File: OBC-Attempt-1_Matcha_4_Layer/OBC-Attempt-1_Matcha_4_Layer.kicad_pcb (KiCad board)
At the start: 4 copper layers, 57.1 x 57.1 mm, 76 parts, among them J1 Screw_Terminal_01x08, J2 Screw_Terminal_01x08, J3 USB_B_Micro, J4 Screw_Terminal_01x08, J5 Conn_01x04, J6 Micro_SD_Card, J7 Screw_Terminal_01x02, J8 Screw_Terminal_01x02, Q1 2N7002K, Q2 2N7002K, Q3 2N7002K, Q4 2N7002K, SW1 PCM12SMTR, U1 BMI088, U10 CPC1020NTR, U11 CPC1020NTR, U12 NCP1117-3.3_SOT223, U2 CPC1020NTR, U3 CPC1020NTR, U4 CPC1020NTR, U5 CPC1020NTR, U6 NCP1117-3.3_SOT223, U7 CPC1020NTR, U8 CPC1020NTR, U9 STM32F401RDTx, Y1 ABMM2-25MHZ-D1-T

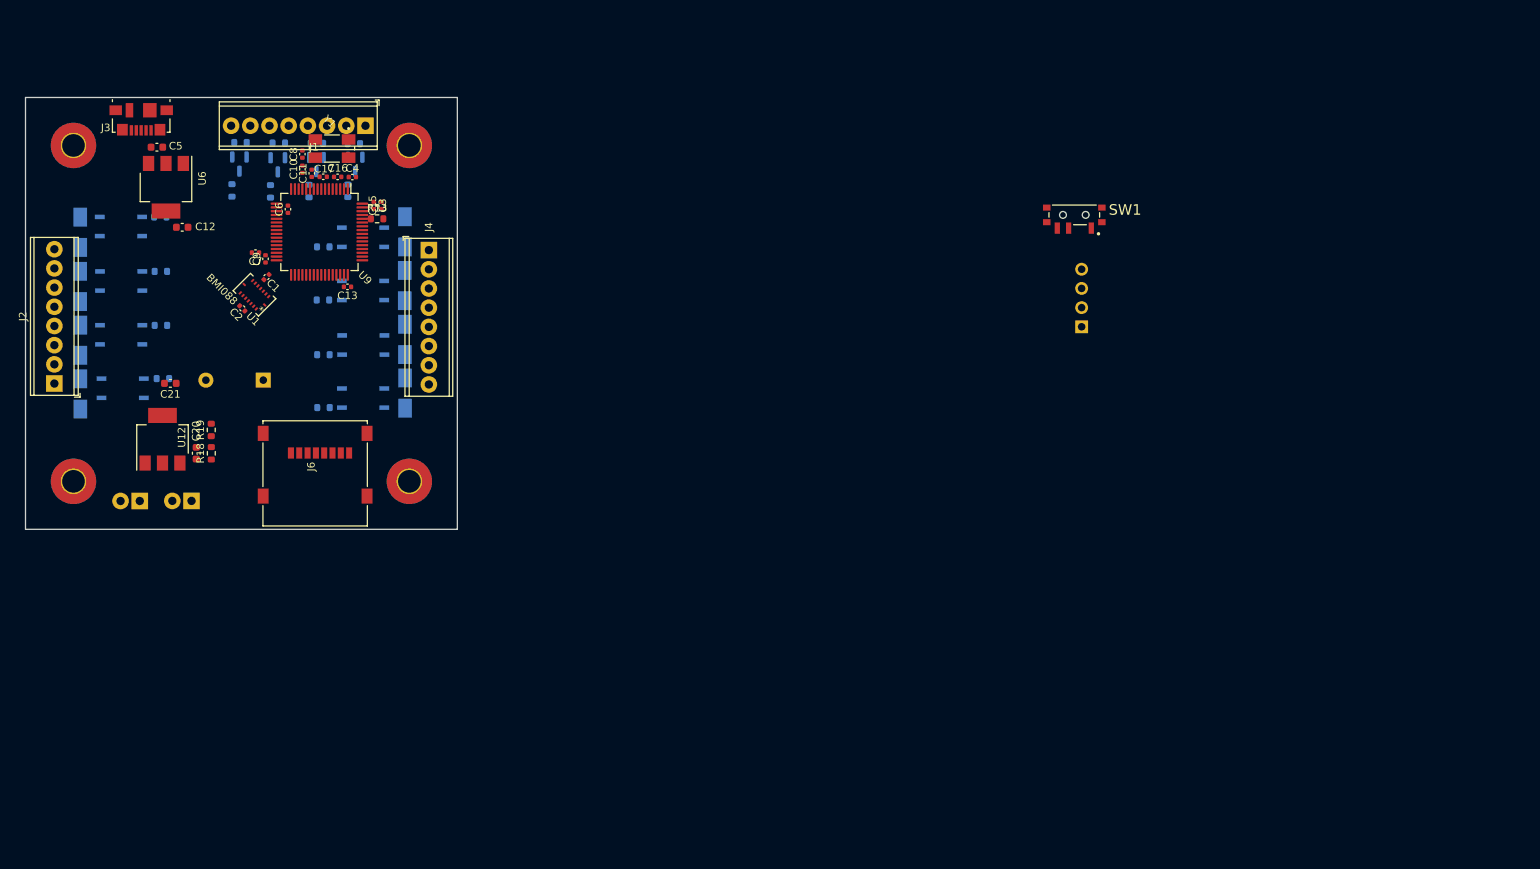
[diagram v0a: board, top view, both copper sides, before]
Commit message: start over
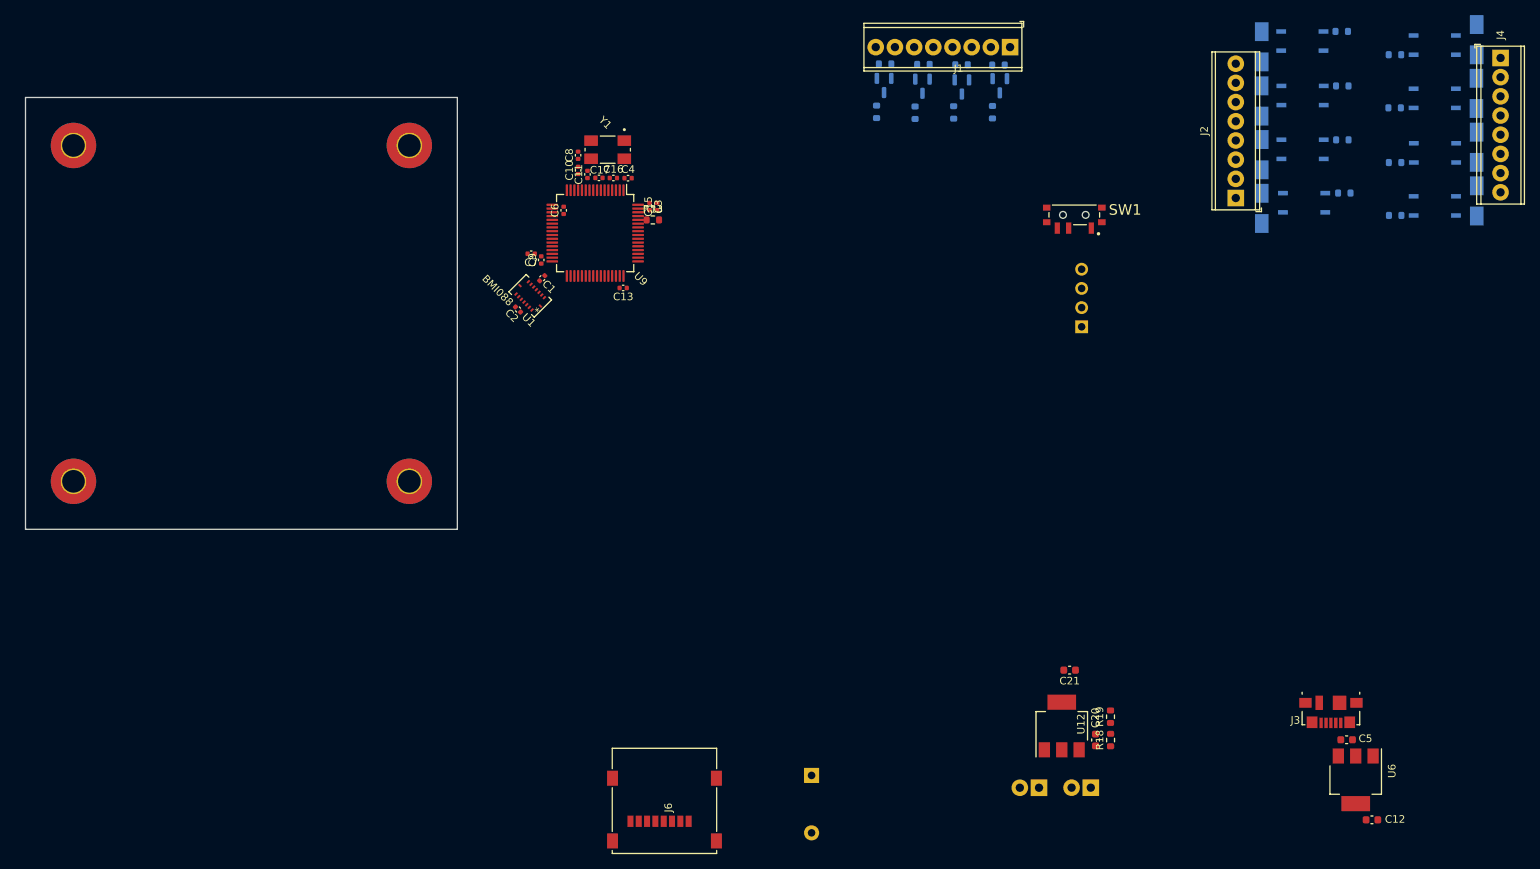
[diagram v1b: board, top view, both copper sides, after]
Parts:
- moved C5 175.9 mm to (200.2, 110.4)
- moved C12 175.9 mm to (203.6, 121.0)
- moved J3 175.9 mm to (198.2, 106.7)
- moved U6 175.9 mm to (201.4, 115.7)
- moved D4 158.3 mm to (189.0, 25.9)
- moved R11 158.3 mm to (199.9, 38.0)
- moved R9 158.3 mm to (199.7, 31.0)
- moved U4 158.3 mm to (194.6, 39.3)
- moved D1 158.3 mm to (189.0, 40.1)
- moved D2 158.3 mm to (189.0, 18.7)
- moved D3 158.3 mm to (189.0, 33.0)
- moved J2 158.3 mm to (185.6, 38.7)
- moved R10 158.3 mm to (199.7, 23.9)
- moved R12 158.3 mm to (199.6, 16.7)
- moved U2 158.3 mm to (194.4, 32.3)
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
